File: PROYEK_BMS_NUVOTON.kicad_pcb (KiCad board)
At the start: 2 copper layers, 95.9 x 107.3 mm, 256 parts, among them J1 Conn_01x23_Pin, J2 Conn_01x04_Pin, J3 USB_B_Micro, J4 Screw_Terminal_01x02, Q1 NPN, Q10 Q_NMOS_GSD, Q11 Q_NMOS_GSD, Q12 Q_NMOS_GSD, Q13 Q_NMOS_GSD, Q14 Q_NMOS_GSD, Q15 Q_NMOS_GSD, Q16 Q_NMOS_GSD, Q17 Q_NMOS_GSD, Q18 Q_NMOS_GSD, Q19 Q_NMOS_GSD, Q2 Q_NMOS_GSD, Q20 Q_NMOS_GSD, Q21 Q_NMOS_GSD, Q22 Q_NMOS_GSD, Q23 Q_NMOS_GSD, Q24 NMOS, Q25 NMOS, Q26 NMOS, Q27 NMOS, Q28 NMOS, Q29 NMOS, Q3 Q_NMOS_GSD, Q30 NMOS, Q31 NMOS, Q32 NMOS, Q33 NMOS, Q34 NMOS, Q35 NMOS, Q4 Q_NMOS_GSD, Q5 Q_NMOS_GSD, Q6 Q_NMOS_GSD, Q7 Q_NMOS_GSD, Q8 Q_NMOS_GSD, Q9 Q_NMOS_GSD, SW1 SW_SPDT, SW2 SW_Push, SW3 SW_SPDT, U2 TL431DBZ, U3 TL431DBZ, U4 STM32F072RBTx, U5 SN65HVD230, U6 AP7370-33SA-7, Y1 8M,SMD, Y2 32.768k,SMD

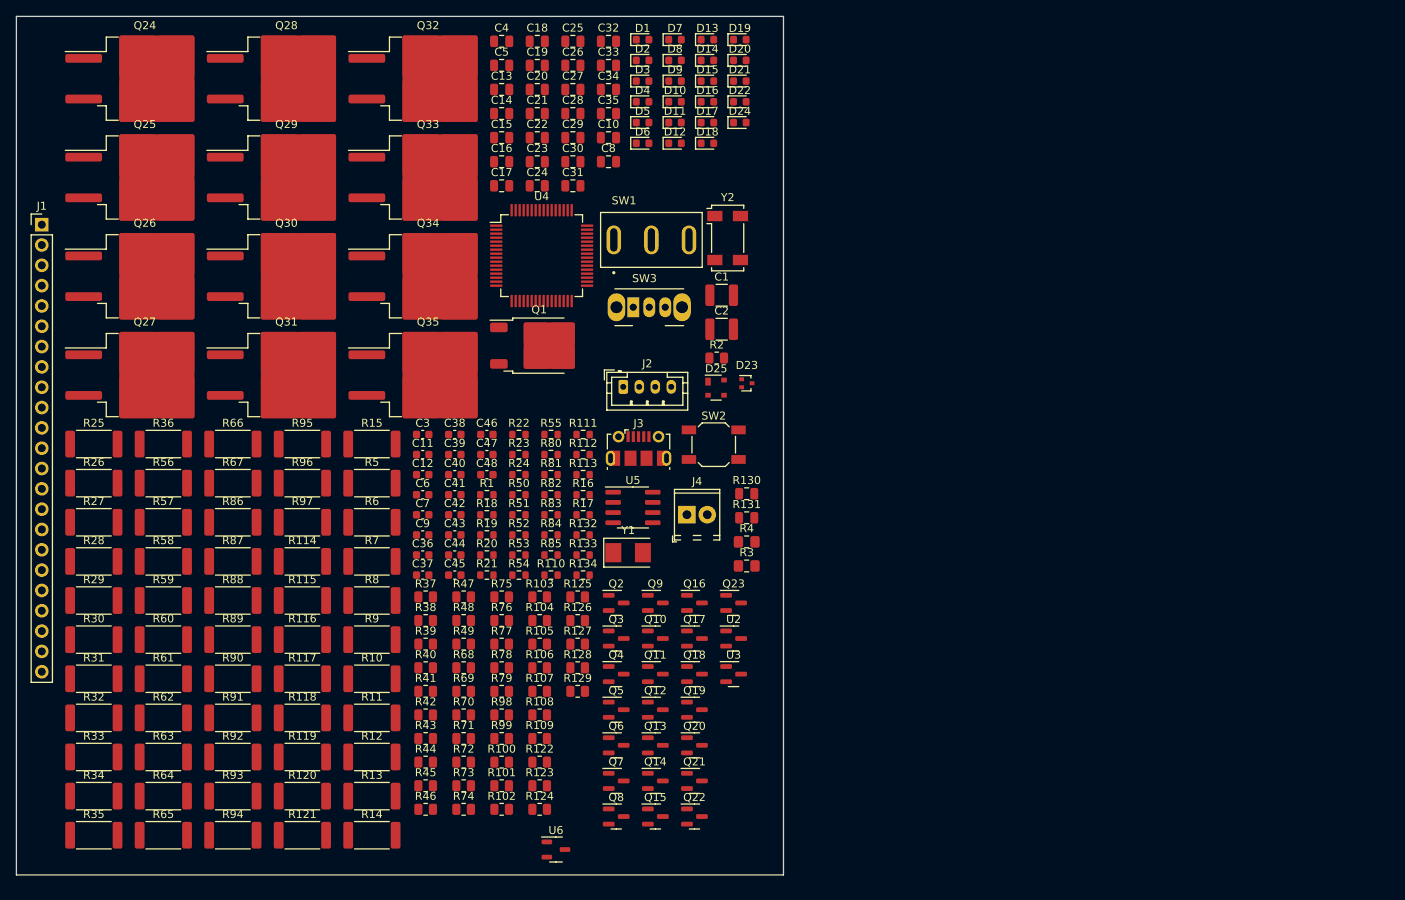
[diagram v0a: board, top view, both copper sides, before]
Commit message: revision 7 March
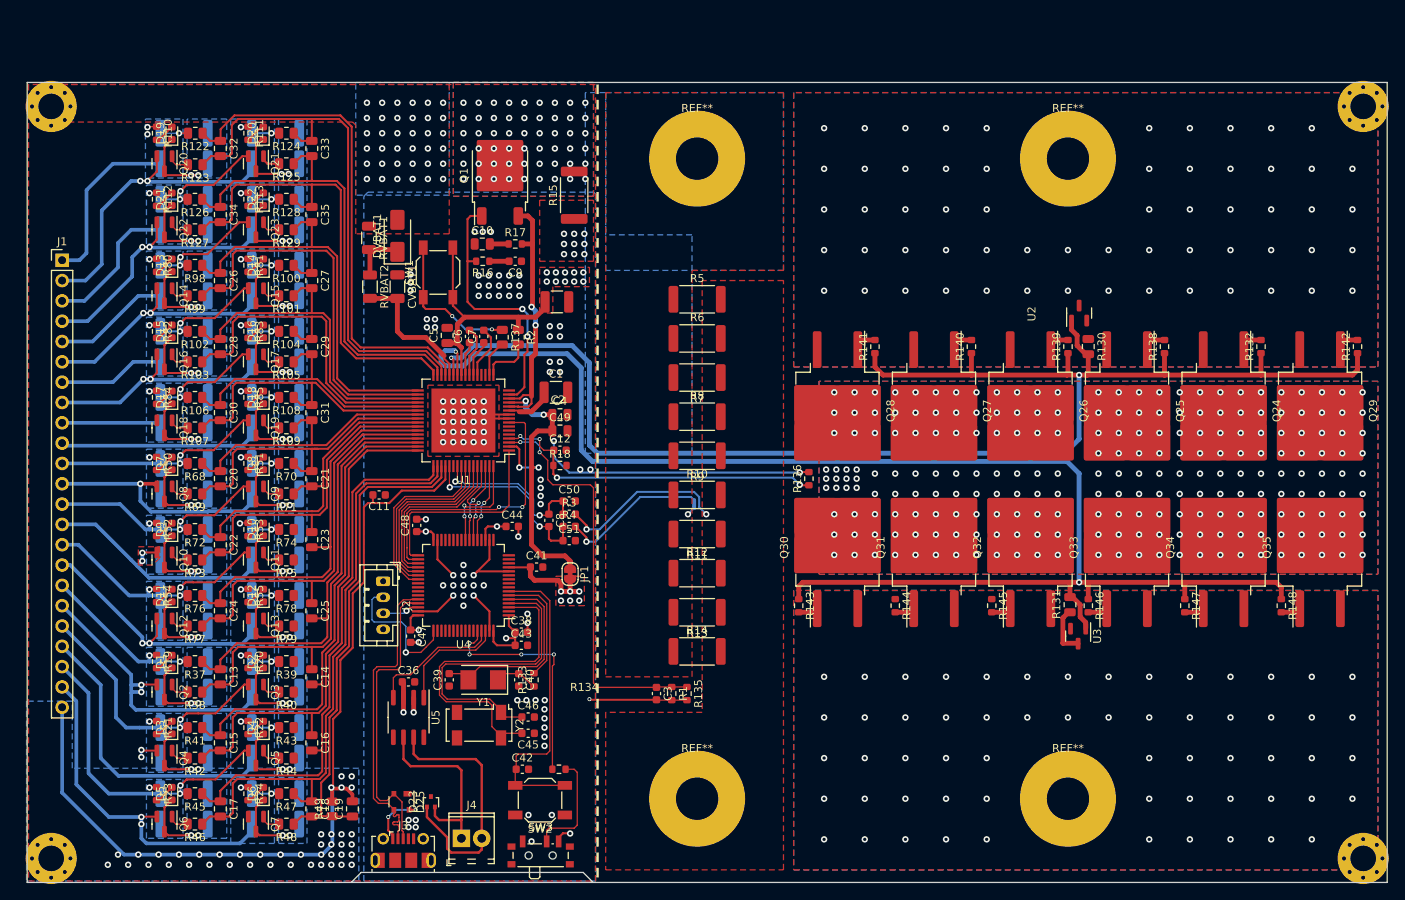
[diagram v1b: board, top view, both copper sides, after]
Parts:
- removed C37: 1u,0603, Capacitor_SMD:C_0603_1608Metric
- removed D24: GREEN_LED, LED_SMD:LED_0603_1608Metric
- removed U6: AP7370-33SA-7, Package_TO_SOT_SMD:SOT-23-3
- added C49: 0.1 uF, Capacitor_SMD:C_0805_2012Metric, F.Cu at (127.0, 89.9)
- added C50: 0.1u, Capacitor_SMD:C_0603_1608Metric, F.Cu at (128.2, 98.7)
- added C51: 0.1u, Capacitor_SMD:C_0603_1608Metric, F.Cu at (128.2, 103.6)
- added CVBAT1: 1uF, Capacitor_SMD:C_1206_3216Metric, F.Cu at (106.7, 71.9)
- added DVBAT1: US1M, Diode_SMD:D_SMA, F.Cu at (106.7, 65.5)
- added JP1: Jumper_2_Bridged, Jumper:SolderJumper-2_P1.3mm_Bridged_RoundedPad1.0x1.5mm, F.Cu at (128.3, 107.8)
- added NT1: NetTie_2, NetTie:NetTie-2_SMD_Pad0.5mm, B.Cu at (143.8, 99.1)
- added R135: NTC10k, Resistor_SMD:R_0603_1608Metric, F.Cu at (142.9, 122.7)
- added R136: NTC10k, Resistor_SMD:R_0603_1608Metric, F.Cu at (158.1, 95.9)
- added R137: 75M, Resistor_SMD:R_0805_2012Metric, F.Cu at (119.8, 78.2)
- added R138: 2R2, Resistor_SMD:R_0603_1608Metric, F.Cu at (202.6, 79.4)
- added R139: 2R2, Resistor_SMD:R_0603_1608Metric, F.Cu at (190.5, 79.4)
- added R140: 2R2, Resistor_SMD:R_0603_1608Metric, F.Cu at (178.4, 79.4)
- added R141: 2R2, Resistor_SMD:R_0603_1608Metric, F.Cu at (166.4, 79.4)
- added R142: 2R2, Resistor_SMD:R_0603_1608Metric, F.Cu at (226.7, 79.4)
- added R143: 2R2, Resistor_SMD:R_0603_1608Metric, F.Cu at (156.8, 111.8)
- added R144: 2R2, Resistor_SMD:R_0603_1608Metric, F.Cu at (168.9, 111.8)
- added R145: 2R2, Resistor_SMD:R_0603_1608Metric, F.Cu at (181.0, 111.8)
- added R146: 2R2, Resistor_SMD:R_0603_1608Metric, F.Cu at (193.0, 111.8)
- added R147: 2R2, Resistor_SMD:R_0603_1608Metric, F.Cu at (205.1, 111.8)
- added R148: 2R2, Resistor_SMD:R_0603_1608Metric, F.Cu at (217.2, 111.8)
- added REF**: MountingHole_5.3mm_M5_Pad, MountingHole:MountingHole_5.3mm_M5_Pad, F.Cu at (144.1, 55.9)
- added REF**: MountingHole_5.3mm_M5_Pad, MountingHole:MountingHole_5.3mm_M5_Pad, F.Cu at (190.5, 135.9)
- added REF**: MountingHole_3.2mm_M3_Pad_Via, MountingHole:MountingHole_3.2mm_M3_Pad_Via, F.Cu at (227.4, 49.4)
- added REF**: MountingHole_3.2mm_M3_Pad_Via, MountingHole:MountingHole_3.2mm_M3_Pad_Via, F.Cu at (63.4, 143.4)
- added REF**: MountingHole_3.2mm_M3_Pad_Via, MountingHole:MountingHole_3.2mm_M3_Pad_Via, F.Cu at (63.4, 49.4)
- added REF**: MountingHole_5.3mm_M5_Pad, MountingHole:MountingHole_5.3mm_M5_Pad, F.Cu at (190.5, 55.9)
- added REF**: MountingHole_5.3mm_M5_Pad, MountingHole:MountingHole_5.3mm_M5_Pad, F.Cu at (144.1, 135.9)
- added REF**: MountingHole_3.2mm_M3_Pad_Via, MountingHole:MountingHole_3.2mm_M3_Pad_Via, F.Cu at (227.4, 143.4)
- added RVBAT1: 100, Resistor_SMD:R_1206_3216Metric, F.Cu at (103.1, 65.8)
- added RVBAT2: 100, Resistor_SMD:R_1206_3216Metric, F.Cu at (103.3, 71.9)
- added U1: KA49522, Package_QFP:HTQFP-64-1EP_10x10mm_P0.5mm_EP8x8mm, F.Cu at (114.9, 88.6)
- C1: value 2.2u -> 4.7u
- C12, C3: value 100n -> 1n
- C36: value 1u,0603 -> 100n,0603
- C8: footprint Capacitor_SMD:C_0805_2012Metric -> Capacitor_SMD:C_0603_1608Metric
- R1: value NTC10k -> 47k
- R114, R115, R116, R117, R118, R119, R120, R121, R25, R26, R27, R28, R29, R30, R31, R32, R33, R34, R35, R36, R56, R57, R58, R59, R60, R61, R62, R63, R64, R65, R66, R67, R86, R87, R88, R89, R90, R91, R92, R93, R94, R95, R96, R97: moved to B.Cu
- R132: value 1.2k,0603 -> 2R2
- R18: value R -> 47k
- R2: value 100 -> 30k
- R3, R4: footprint Capacitor_SMD:C_0805_2012Metric_Pad1.18x1.45mm_HandSolder -> Capacitor_SMD:C_0603_1608Metric
- SW1: value SW_SPDT -> SW_Push; footprint PROYEK_BMS_NUVOTON:SW_100SP1T1B1M1QEH -> Button_Switch_SMD:SW_SPST_SKQG_WithStem
- SW3: footprint Button_Switch_THT:SW_CuK_OS102011MA1QN1_SPDT_Angled -> Button_Switch_SMD:SW_SPDT_PCM12
- moved Q24 141.1 mm to (209.9, 87.4), turned to -90 degrees
- moved Q29 132.5 mm to (222.0, 87.4), turned to -90 degrees
- moved Q25 126.2 mm to (197.9, 87.4), turned to -90 degrees
- moved Q35 113.6 mm to (222.0, 104.5), turned to 90 degrees
- moved Q26 112.0 mm to (185.8, 87.4), turned to -90 degrees
- moved Q34 105.1 mm to (209.9, 104.5), turned to 90 degrees
- moved D5 102.5 mm to (78.5, 135.3), turned to 90 degrees
- moved C18 100.0 mm to (96.0, 137.2), turned to -90 degrees
- moved D3 100.0 mm to (78.5, 127.0), turned to 90 degrees
- moved Q33 98.9 mm to (197.9, 104.5), turned to 90 degrees
- moved Q22 98.8 mm to (77.6, 64.8), turned to -90 degrees
- moved Q27 98.7 mm to (173.8, 87.4), turned to -90 degrees
- moved Q20 98.4 mm to (77.6, 56.5), turned to -90 degrees
- moved D1 97.5 mm to (78.5, 118.7), turned to 90 degrees
- moved C19 95.8 mm to (101.1, 137.2), turned to 90 degrees
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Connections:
- C1 pad 2: CN4_C0 -> GND
- C10 pad 1: CN4_C0 -> GND
- C11 pad 1: CN4_C0 -> C0
- C11 pad 2: C0 -> GND
- C12 pad 1: TMON1 -> TMON2
- C12 pad 2: CN4_C0 -> GND
- C19 pad 2: GNDA -> GND
- C2 pad 2: CN4_C0 -> GND
- C3 pad 1: TMON2 -> TMON1
- C3 pad 2: CN4_C0 -> GND
- C36 pad 1: +5V -> +3V3
- C36 pad 2: CN4_C0 -> GND
- C38 pad 2: CN4_C0 -> GND
- C39 pad 1: CN4_C0 -> GND
- C39 pad 2: /OSC_0_IN -> /OSC_IN
- C4 pad 1: BMS_5V -> BMS_3.3V
- C4 pad 2: CN4_C0 -> GND
- C40 pad 2: CN4_C0 -> GND
- C41 pad 2: CN4_C0 -> GND
- C42 pad 2: CN4_C0 -> GND
- C43 pad 2: CN4_C0 -> GND
- C44 pad 2: CN4_C0 -> GND
- C45 pad 1: CN4_C0 -> GND
- C46 pad 2: CN4_C0 -> GND
- C47 pad 2: CN4_C0 -> GND
- C48 pad 2: CN4_C0 -> GND
- C5 pad 2: CN4_C0 -> GND
- C9 pad 1: CN4_C0 -> GND
- D23 pad 3: CN4_C0 -> GND
- D25 pad 1: CN4_C0 -> GND
- D25 pad 4: +5V -> USB_5V
- J1 pad 23: CN4_C0 -> GND
- J2 pad 1: CN4_C0 -> GND
- J3 pad 5: CN4_C0 -> GND
- J4 pad 1: /CAN_D+ -> /CAN_D-
- J4 pad 2: /CAN_D- -> /CAN_D+
- Q1 pad 1: Net-(Q1-C) -> REGB
- Q1 pad 2: REGB -> Net-(Q1-C)
- Q24 pad 1: REG_SUP -> Net-(Q24-G)
- Q24 pad 2: CHG -> REG_SUP
- Q25 pad 1: REG_SUP -> Net-(Q25-G)
- Q25 pad 2: CHG -> REG_SUP
- Q26 pad 1: REG_SUP -> Net-(Q26-G)
- Q26 pad 2: CHG -> REG_SUP
- Q27 pad 1: REG_SUP -> Net-(Q27-G)
- Q27 pad 2: CHG -> REG_SUP
- Q28 pad 1: REG_SUP -> Net-(Q28-G)
- Q28 pad 2: CHG -> REG_SUP
- Q29 pad 1: REG_SUP -> Net-(Q29-G)
- Q29 pad 2: CHG -> REG_SUP
- Q30 pad 1: REG_SUP -> Net-(Q30-G)
- Q30 pad 2: DIS -> REG_SUP
- Q31 pad 1: REG_SUP -> Net-(Q31-G)
- Q31 pad 2: DIS -> REG_SUP
- Q32 pad 1: REG_SUP -> Net-(Q32-G)
- Q32 pad 2: DIS -> REG_SUP
- Q33 pad 1: REG_SUP -> Net-(Q33-G)
- Q33 pad 2: DIS -> REG_SUP
- Q34 pad 1: REG_SUP -> Net-(Q34-G)
- Q34 pad 2: DIS -> REG_SUP
- Q35 pad 1: REG_SUP -> Net-(Q35-G)
- Q35 pad 2: DIS -> REG_SUP
- Q7 pad 2: CN4_C0 -> GND
- R1 pad 1: TMON2 -> TMON1
- R1 pad 2: CN4_C0 -> GND
- R10 pad 1: CN4_C0 -> GND
- R11 pad 1: CN4_C0 -> VPACK-
- R11 pad 2: VPACK- -> GND
- R12 pad 1: CN4_C0 -> GND
- R13 pad 1: CN4_C0 -> VPACK-
- R13 pad 2: VPACK- -> GND
- R132 pad 1: CN4_C0 -> CHG
- R132 pad 2: Net-(D24-K) -> Net-(Q24-G)
- R133 pad 2: /OSC_0_OUT -> /OSC_OUT
- R14 pad 1: CN4_C0 -> GND
- R18 pad 1: TMON1 -> TMON2
- R18 pad 2: CN4_C0 -> GND
- R4 pad 2: CN4_C0 -> Net-(NT1-Pad2)
- R49 pad 2: CN4_C0 -> GND
- R5 pad 1: CN4_C0 -> GND
- R55 pad 1: unconnected-(R55-Pad1) -> CN4_C7
- R6 pad 1: CN4_C0 -> GND
- R7 pad 1: CN4_C0 -> VPACK-
- R7 pad 2: VPACK- -> GND
- R8 pad 1: CN4_C0 -> GND
- R9 pad 1: CN4_C0 -> VPACK-
- R9 pad 2: VPACK- -> GND
- SW1 pad 1: BMS_5V -> Net-(R137-Pad1)
- SW1 pad 2: +5V -> VPACK+
- SW2 pad 1: CN4_C0 -> GND
- SW3 pad 1: CN4_C0 -> GND
- U4 pad 12: CN4_C0 -> GND
- U4 pad 18: CN4_C0 -> GND
- U4 pad 3: /OSC32_OUT -> /OSC32_IN
- U4 pad 31: CN4_C0 -> GND
- U4 pad 47: CN4_C0 -> GND
- U4 pad 63: CN4_C0 -> GND
- U5 pad 2: CN4_C0 -> GND
- U5 pad 8: CN4_C0 -> GND
- Y1 pad 2: /OSC_0_IN -> /OSC_IN
- Y2 pad 2: /OSC32_IN -> unconnected-(Y2-Pad2)
- Y2 pad 3: (no net) -> unconnected-(Y2-Pad3)
- Y2 pad 4: (no net) -> /OSC32_IN
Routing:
- net GND: track 0.00 -> 203.7 mm, vias 0 -> 145
- net DIS: track 0.00 -> 187.3 mm, vias 0 -> 2
- net CHG: track 0.00 -> 185.5 mm, vias 0 -> 2
- net C1: track 0.00 -> 74.5 mm
- net C21: track 0.00 -> 69.1 mm
- net C2: track 0.00 -> 67.6 mm
- net C3: track 0.00 -> 63.5 mm
- net C22: track 0.00 -> 62.6 mm
- net C0: track 0.00 -> 62.4 mm
- net C19: track 0.00 -> 60.3 mm
- net C4: track 0.00 -> 60.1 mm
- net C20: track 0.00 -> 59.7 mm
- net C5: track 0.00 -> 56.6 mm
- net C6: track 0.00 -> 53.8 mm
- net C17: track 0.00 -> 53.4 mm
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- added copper zone on F.Cu, net +3V3
- added copper zone on In2.Cu, net +3V3
- added copper zone on B.Cu, net CN4_C1
- added copper zone on B.Cu, net CN4_C10
- added copper zone on B.Cu, net CN4_C11
- added copper zone on B.Cu, net CN4_C12
- added copper zone on B.Cu, net CN4_C13
- added copper zone on B.Cu, net CN4_C14
- added copper zone on B.Cu, net CN4_C15
- added copper zone on B.Cu, net CN4_C16
- added copper zone on B.Cu, net CN4_C17
- added copper zone on B.Cu, net CN4_C18
- added copper zone on B.Cu, net CN4_C19
- added copper zone on B.Cu, net CN4_C2
- added copper zone on B.Cu, net CN4_C20
- added copper zone on B.Cu, net CN4_C21
- added copper zone on B.Cu, net CN4_C22
- added copper zone on F.Cu, net CN4_C22
- added copper zone on In1.Cu, net CN4_C22
- added copper zone on In2.Cu, net CN4_C22
- added copper zone on B.Cu, net CN4_C3
- added copper zone on B.Cu, net CN4_C4
- added copper zone on B.Cu, net CN4_C5
- added copper zone on B.Cu, net CN4_C6
- added copper zone on B.Cu, net CN4_C7
- added copper zone on B.Cu, net CN4_C8
- added copper zone on B.Cu, net CN4_C9
- added copper zone on F.Cu, net CN4_C9
- added copper zone on B.Cu, net GND
- added copper zone on F.Cu, net GND
- added copper zone on In1.Cu, net GND
- added copper zone on B.Cu, net Net-(D1-K)
- added copper zone on B.Cu, net Net-(D10-K)
- added copper zone on B.Cu, net Net-(D11-K)
- added copper zone on B.Cu, net Net-(D12-K)
- added copper zone on B.Cu, net Net-(D13-K)
- added copper zone on B.Cu, net Net-(D14-K)
- added copper zone on B.Cu, net Net-(D15-K)
- added copper zone on B.Cu, net Net-(D16-K)
- added copper zone on B.Cu, net Net-(D17-K)
- added copper zone on B.Cu, net Net-(D18-K)
- added copper zone on B.Cu, net Net-(D19-K)
- added copper zone on B.Cu, net Net-(D2-K)
- added copper zone on B.Cu, net Net-(D20-K)
- added copper zone on B.Cu, net Net-(D21-K)
- added copper zone on B.Cu, net Net-(D22-K)
- added copper zone on B.Cu, net Net-(D3-K)
- added copper zone on B.Cu, net Net-(D4-K)
- added copper zone on B.Cu, net Net-(D5-K)
- added copper zone on B.Cu, net Net-(D6-K)
- added copper zone on B.Cu, net Net-(D7-K)
- added copper zone on B.Cu, net Net-(D8-K)
- added copper zone on B.Cu, net Net-(D9-K)
- added copper zone on B.Cu, net Net-(Q1-C)
- added copper zone on F.Cu, net Net-(Q1-C)
- added copper zone on In1.Cu, net Net-(Q1-C)
- added copper zone on In2.Cu, net Net-(Q1-C)
- added copper zone on B.Cu, net REG_SUP
- added copper zone on F.Cu, net REG_SUP
- added copper zone on In1.Cu, net REG_SUP
- added copper zone on In2.Cu, net REG_SUP
- added copper zone on B.Cu, net VPACK+
- added copper zone on F.Cu, net VPACK+
- added copper zone on In1.Cu, net VPACK+
- added copper zone on In2.Cu, net VPACK+
- added copper zone on F.Cu, net VPACK-
- added copper zone on In1.Cu, net VPACK-
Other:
- board size 95.9 x 107.3 mm -> 170 x 100 mm
- copper layers 2 -> 4
